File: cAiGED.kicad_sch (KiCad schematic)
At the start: 0 parts

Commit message: Updated project files
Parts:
- added IC1: STM32N657X0H3Q, BGA264C80P17X17_1400X1400X100, symbol SamacSys_Parts3:STM32N657X0H3Q

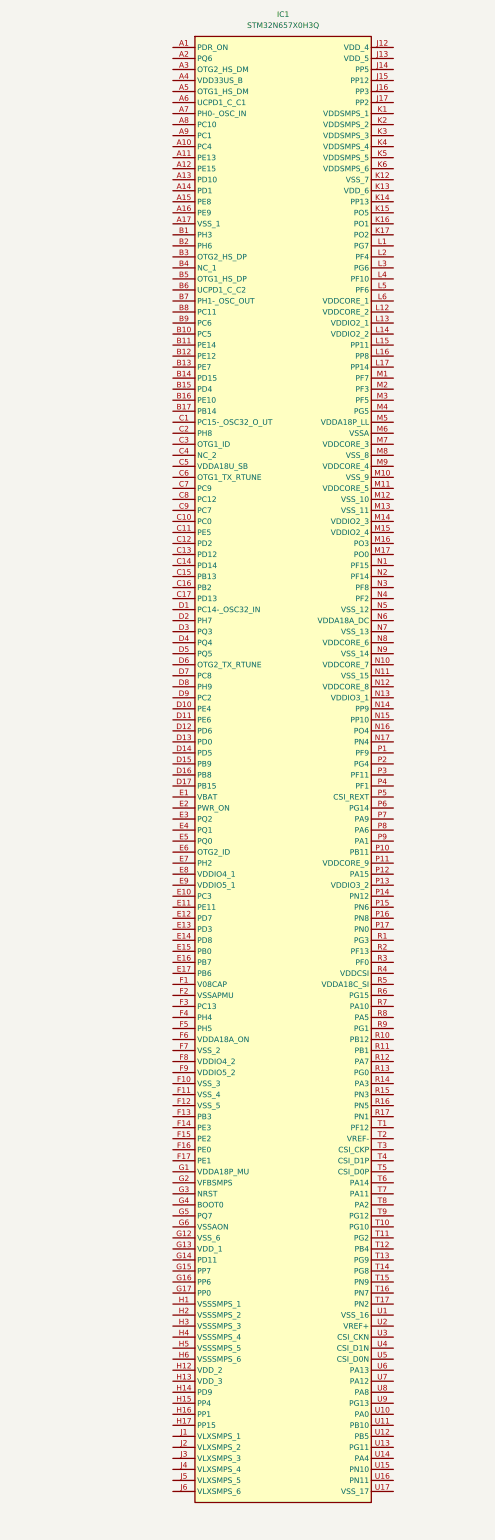
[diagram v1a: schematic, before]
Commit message: Updated Documentation files. Updated MCU symbol
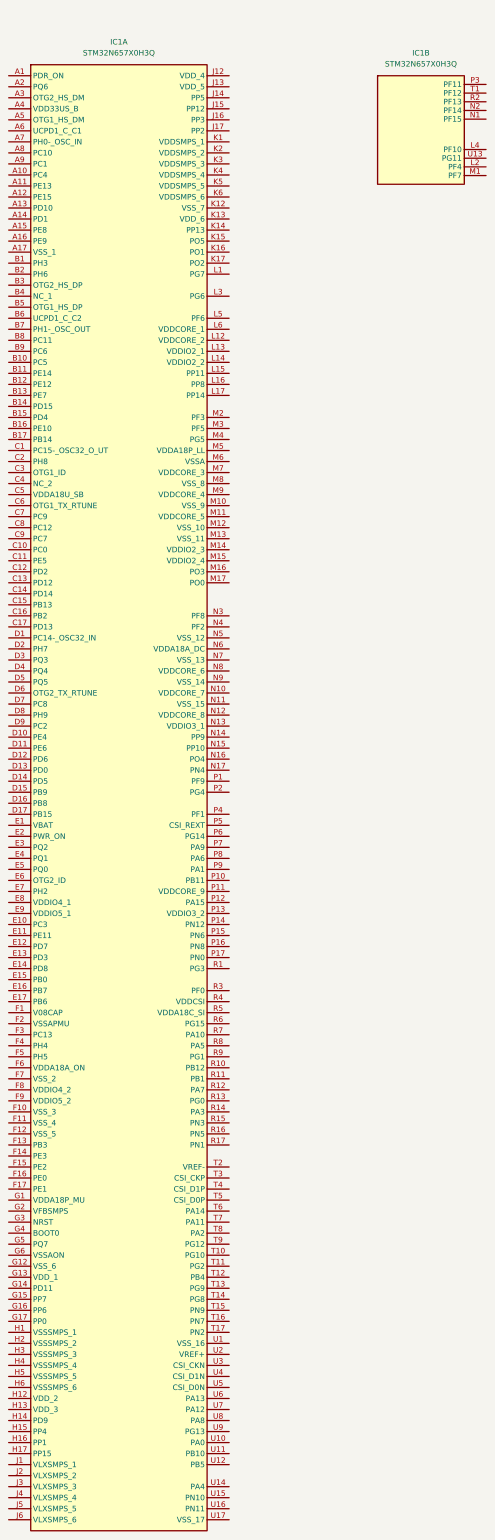
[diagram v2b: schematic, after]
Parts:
- added unit 2 of IC1
